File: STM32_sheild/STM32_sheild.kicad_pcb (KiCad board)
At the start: 2 copper layers, 70 x 67 mm, 48 parts, among them J1 61612002121503, J2 CN7, J3 CN10, J4 632722100213, J5 691210910002, J6 691210910002, U1 OPA333xxDBV, U2 TPS63031DSK, U3 MCP73831-2-MC, U4 OPA333xxDBV

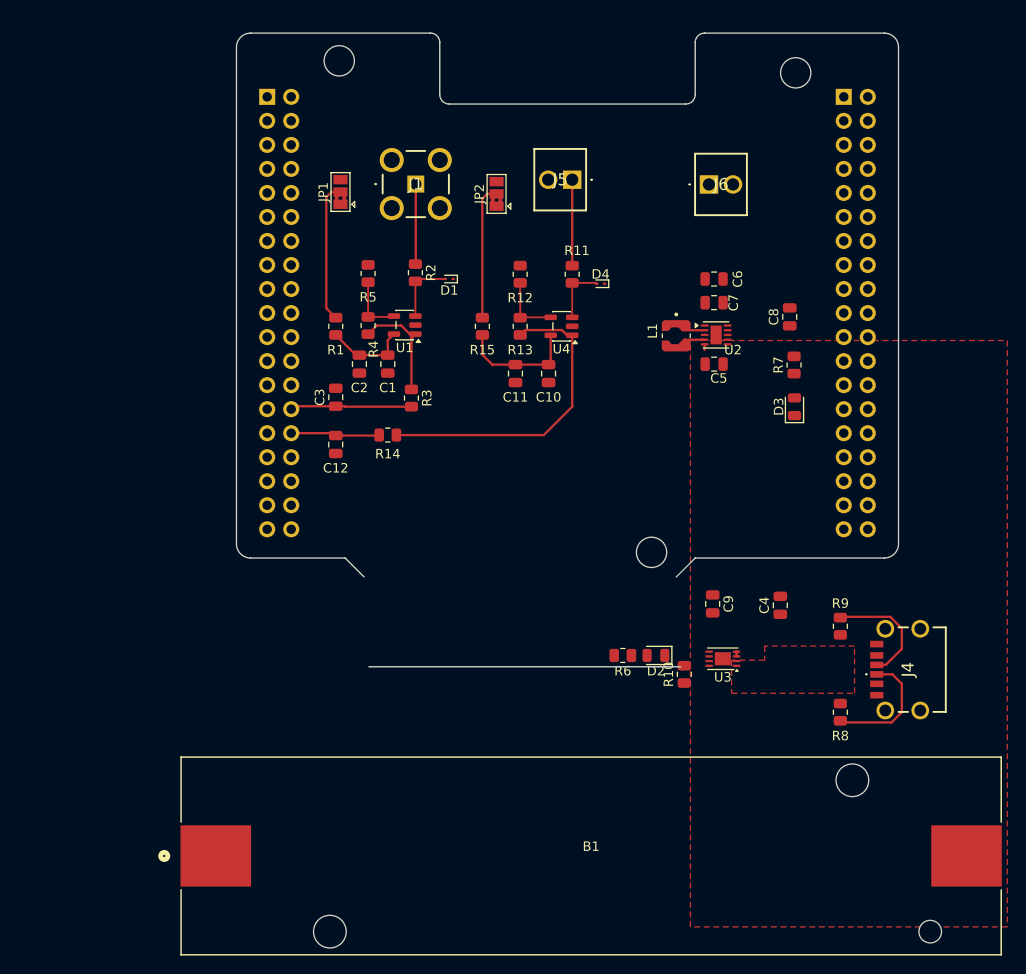
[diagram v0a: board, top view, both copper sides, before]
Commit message: Added mulitple pours in layout
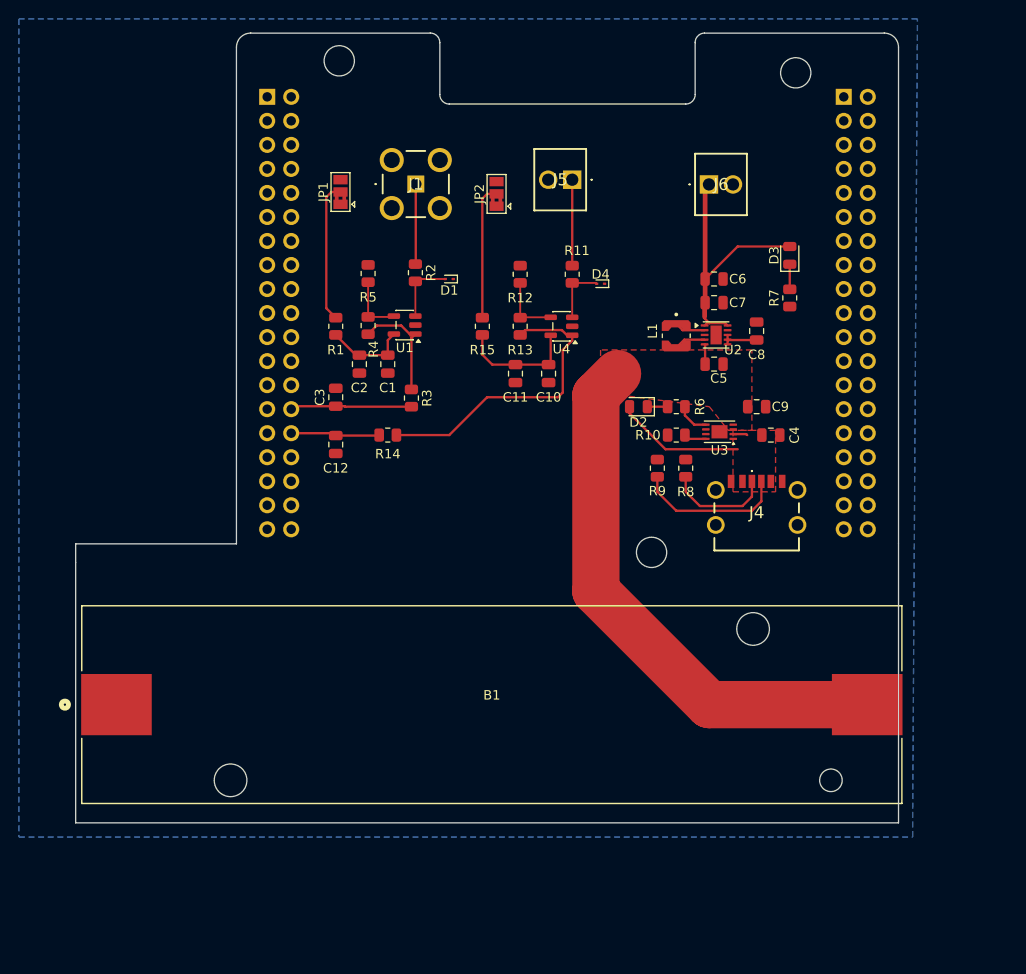
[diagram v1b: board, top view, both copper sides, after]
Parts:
- moved R8 30.5 mm to (149.0, 101.5)
- moved R6 26.9 mm to (148.0, 95.0)
- moved D2 26.4 mm to (144.0, 95.0)
- moved R9 25.6 mm to (146.0, 101.5), turned to 90 degrees
- moved R10 25.3 mm to (148.0, 98.0), turned to 180 degrees
- moved U3 24.0 mm to (152.6, 97.7)
- moved J4 23.1 mm to (156.5, 106.5), turned to 0 degrees
- moved C9 21.4 mm to (156.5, 95.0), turned to 0 degrees
- moved B1 19.1 mm to (128.5, 126.5)
- moved C4 18.0 mm to (158.0, 98.0), turned to 0 degrees
- moved D3 16.0 mm to (160.0, 79.0)
- moved R7 7.10 mm to (160.0, 83.5)
- moved C8 3.81 mm to (156.5, 87.0)
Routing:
- net +BATT: track 1.09 -> 59.7 mm
- net +3.3V_REG: track 0.00 -> 28.1 mm
- net V_USB: track 0.35 -> 15.6 mm
- net Net-(U2-EN): track 0.00 -> 4.09 mm
- net Net-(U3-STAT): track 0.00 -> 3.53 mm
- net Net-(J4-CC2): track 12.6 -> 15.9 mm
- net Net-(D3-K): track 0.00 -> 2.65 mm
- net Net-(U3-PROG): track 0.00 -> 2.38 mm
- net Net-(D2-K): track 0.00 -> 2.15 mm
- net Net-(J4-CC1): track 13.1 -> 11.2 mm
- net /OPA2_out: track 33.3 -> 31.9 mm
- added copper zone on B.Cu, net GND
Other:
- board size 70 x 67 mm -> 87 x 83.5 mm
